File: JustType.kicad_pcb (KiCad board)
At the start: 2 copper layers, 152.8 x 109.1 mm, 58 parts, among them J1 Conn_01x02, J2 Conn_01x02, SW1 SW_Push, SW10 SW_Push, SW11 SW_Push, SW12 SW_Push, SW13 SW_Push, SW14 SW_Push, SW15 SW_Push, SW16 SW_Push, SW17 SW_Push, SW18 SW_Push, SW19 SW_Push, SW19'1 SW_Push, SW2 SW_Push, SW20 SW_Push, SW21 SW_Push, SW22 SW_Push, SW23 SW_Push, SW24 SW_Push, SW25 SW_Push, SW3 SW_Push, SW4 SW_Push, SW5 SW_Push, SW6 SW_Push, SW7 SW_Push, SW8 SW_Push, SW9 SW_Push, U1 ProMicro

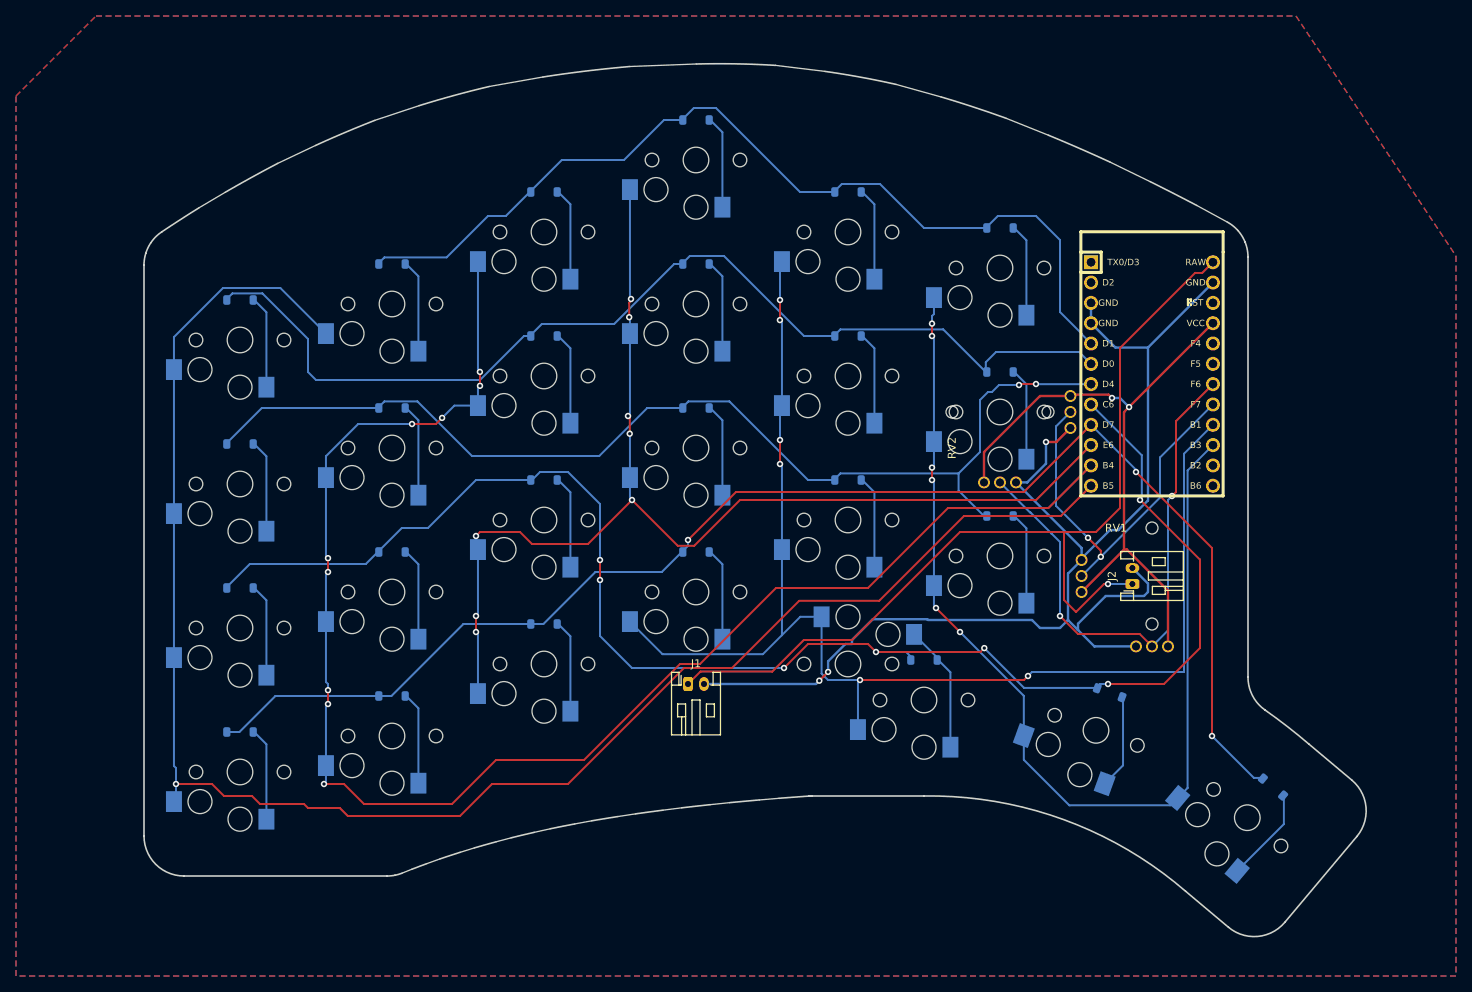
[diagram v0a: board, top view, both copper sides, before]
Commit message: v4
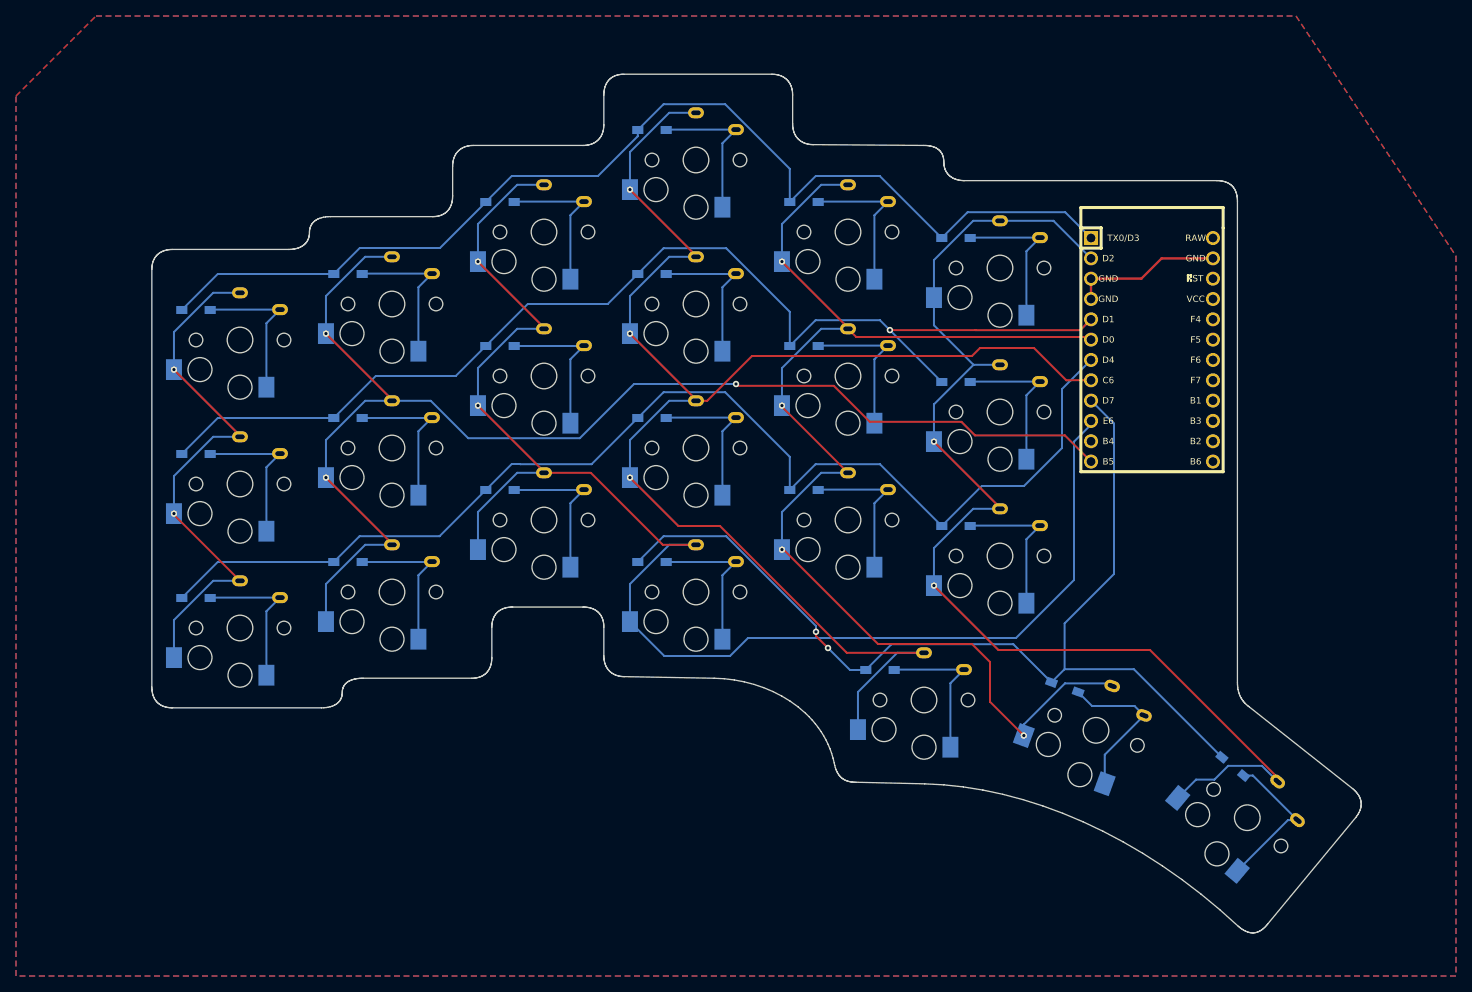
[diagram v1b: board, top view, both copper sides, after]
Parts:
- removed D23, D24, D25: 1N4448W, Diode_SMD:D_SOD-123
- removed J1, J2: Conn_01x02, Connector_JST:JST_PH_S2B-PH-K_1x02_P2.00mm_Horizontal
- removed REF**: KiCad-Logo2_5mm_SilkScreen, Symbol:KiCad-Logo2_5mm_SilkScreen
- removed REF**: OSHW-Logo_5.7x6mm_SilkScreen, Symbol:OSHW-Logo_5.7x6mm_SilkScreen
- removed RV1, RV2: R_Potentiometer_Dual, keyboard_jsa:PSP thumbstick
- removed SW19'1, SW23, SW24, SW25: SW_Push, keyboard_jsa:ChocV1_Hotswap
- D1, D10, D11, D12, D13, D14, D15, D16, D17, D18, D19, D2, D20, D21, D22, D3, D4, D5, D6, D7, D8, D9: footprint Diode_SMD:D_SOD-123 -> keyboard_jsa:D3_SMD_v2
- SW1, SW10, SW11, SW12, SW13, SW14, SW15, SW16, SW17, SW18, SW19, SW2, SW20, SW21, SW22, SW3, SW4, SW5, SW6, SW7, SW8, SW9: footprint keyboard_jsa:ChocV1_Hotswap -> keyboard_jsa:ChocV1_Solder
- moved SW5 101.6 mm to (128.0, 59.5)
- moved D5 96.7 mm to (122.5, 55.8)
- moved SW4 81.7 mm to (109.0, 50.5)
- moved D4 77.0 mm to (103.5, 46.8)
- moved D13 66.9 mm to (46.5, 105.2)
- moved SW10 66.0 mm to (109.0, 68.5)
- moved D10 62.0 mm to (103.5, 64.8)
- moved SW13 61.3 mm to (52.0, 109.0)
- moved SW22 59.4 mm to (177.9, 132.7), turned to 140 degrees
- moved SW21 59.0 mm to (159.0, 121.8), turned to 160 degrees
- moved D21 58.0 mm to (155.1, 116.4), turned to 160 degrees
- moved D22 57.2 mm to (176.1, 126.3), turned to 140 degrees
- moved SW6 57.2 mm to (147.0, 64.0)
- moved D6 51.8 mm to (141.5, 60.2)
- moved SW3 49.4 mm to (90.0, 59.5)
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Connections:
- D10 pad 2: Row 5 -> Row 2
- D11 pad 2: Row 1 -> Row 2
- D14 pad 2: Row 4 -> Row 3
- D15 pad 2: Row 5 -> Row 3
- D16 pad 2: Row 1 -> Row 3
- D17 pad 2: Row 2 -> Row 3
- D2 pad 2: Row 2 -> Row 1
- D20 pad 2: Row 5 -> Row 4
- D21 pad 2: Row 1 -> Row 4
- D22 pad 2: Row 2 -> Row 4
- D3 pad 2: Row 3 -> Row 1
- D4 pad 2: Row 4 -> Row 1
- D5 pad 2: Row 5 -> Row 1
- D8 pad 2: Row 3 -> Row 2
- D9 pad 2: Row 4 -> Row 2
- SW1 pad 1: Col 1 -> Col 6
- SW10 pad 1: Col 2 -> Col 3
- SW11 pad 1: Col 3 -> Col 2
- SW12 pad 1: Col 3 -> Col 1
- SW13 pad 1: Col 3 -> Col 6
- SW14 pad 1: Col 3 -> Col 5
- SW15 pad 1: Col 3 -> Col 4
- SW16 pad 1: Col 4 -> Col 3
- SW17 pad 1: Col 4 -> Col 2
- SW18 pad 1: Col 4 -> Col 1
- SW2 pad 1: Col 1 -> Col 5
- SW20 pad 1: Col 4 -> Col 3
- SW21 pad 1: Col 5 -> Col 2
- SW22 pad 1: Col 5 -> Col 1
- SW3 pad 1: Col 1 -> Col 4
- SW4 pad 1: Col 1 -> Col 3
- SW5 pad 1: Col 1 -> Col 2
- SW6 pad 1: Col 2 -> Col 1
- SW7 pad 1: Col 2 -> Col 6
- SW8 pad 1: Col 2 -> Col 5
- SW9 pad 1: Col 2 -> Col 4
- U1 pad 1: unconnected-(U1-TX0/PD3-Pad1) -> Row 1
- U1 pad 10: Col 3 -> Col 4
- U1 pad 11: Col 2 -> Col 6
- U1 pad 12: Col 1 -> Col 5
- U1 pad 15: Col 5 -> unconnected-(U1-14/PB3-Pad15)
- U1 pad 16: Col 4 -> unconnected-(U1-15/PB1-Pad16)
- U1 pad 17: X -> unconnected-(U1-A0/PF7-Pad17)
- U1 pad 18: Y -> unconnected-(U1-A1/PF6-Pad18)
- U1 pad 2: unconnected-(U1-RX1/PD2-Pad2) -> Col 1
- U1 pad 24: BAT+ -> unconnected-(U1-RAW-Pad24)
- U1 pad 5: Row 1 -> Row 2
- U1 pad 6: Row 2 -> Col 2
- U1 pad 8: Row 4 -> Col 3
- U1 pad 9: Row 5 -> Row 4
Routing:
- net Row 5: track 178.1 -> 0.00 mm, vias 3 -> 0
- net GND: track 161.1 -> 18.8 mm, vias 3 -> 0
- net BAT+: track 118.3 -> 0.00 mm, vias 1 -> 0
- net VCC: track 80.3 -> 0.00 mm, vias 2 -> 0
- net Y: track 69.2 -> 0.00 mm, vias 2 -> 0
- net Col 6: track 0.00 -> 68.4 mm, vias 0 -> 2
- net Col 1: track 215.0 -> 148.2 mm, vias 1 -> 2
- net Row 4: track 194.4 -> 127.9 mm, vias 7 -> 2
- net X: track 49.4 -> 0.00 mm, vias 2 -> 0
- net Col 2: track 195.8 -> 155.9 mm, vias 9 -> 4
- net Col 3: track 146.6 -> 182.9 mm, vias 8 -> 3
- net Col 5: track 130.7 -> 164.4 mm, vias 6 -> 3
- net Row 1: track 116.8 -> 139.5 mm
- net Col 4: track 165.8 -> 187.5 mm, vias 6 -> 2
- net Row 3: track 135.5 -> 149.3 mm, vias 2 -> 0
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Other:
- board size 152.8 x 109.1 mm -> 151.2 x 107.3 mm
- board text added: "Justtype R4 2024-06"
- board text added: "Layout Bold Circuit James"
- board text added: "PRAGMATIC"
- board text removed: "JustType R3 2024-05-11"
- board text removed: "justfont & PRAGMATIC"
- board text removed: "usability bold prototyping james"
- board text removed: "{dblquote}Typography is two-dimensional architecture, based on experience and imagination, and guided by rules and readability.{dblquote} ― Hermann Zapf"
